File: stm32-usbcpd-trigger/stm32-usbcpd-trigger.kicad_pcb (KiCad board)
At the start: 2 copper layers, 24.5 x 13.5 mm, 25 parts, among them J1 USB_C_Receptacle_USB2.0, J2 Conn_01x02_Socket, J3 VBUS, J4 GND, SW1 SW_Push, U1 FUSB302B01MPX, U2 STM32F030F4Px, U3 NCP718

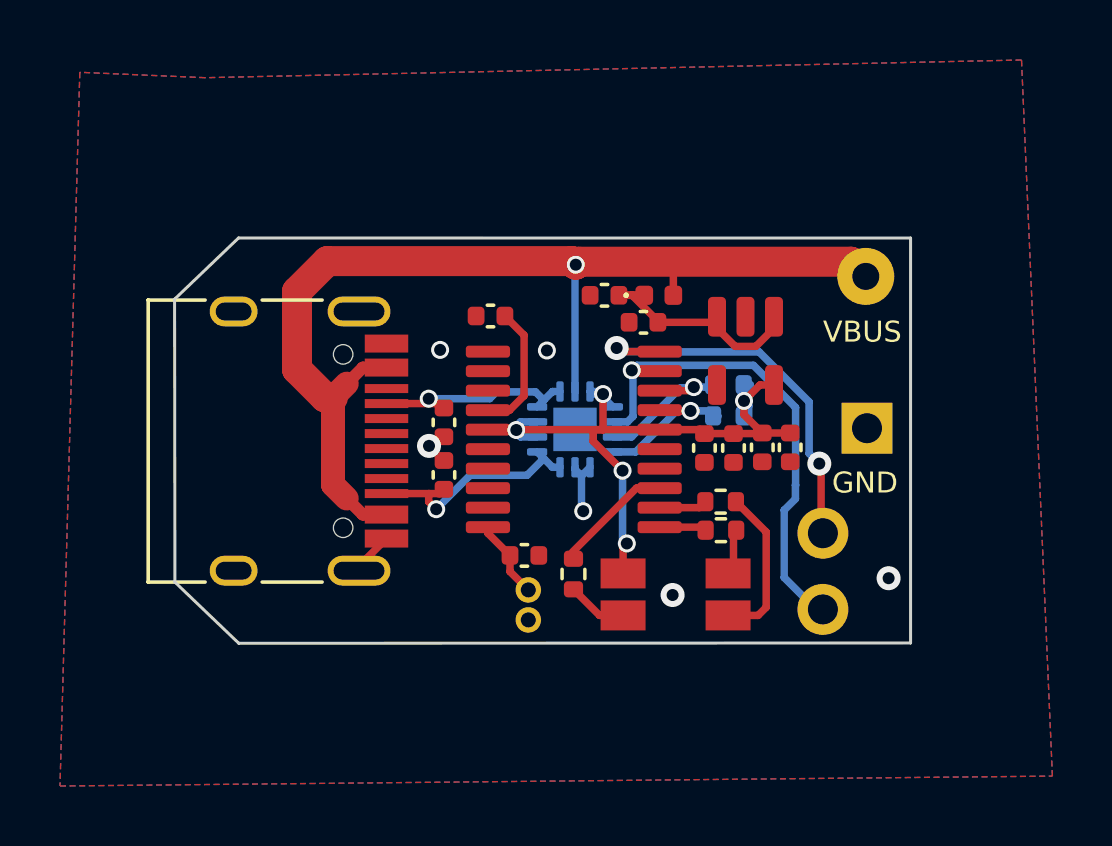
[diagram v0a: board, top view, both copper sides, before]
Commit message: updated stm32 trigger
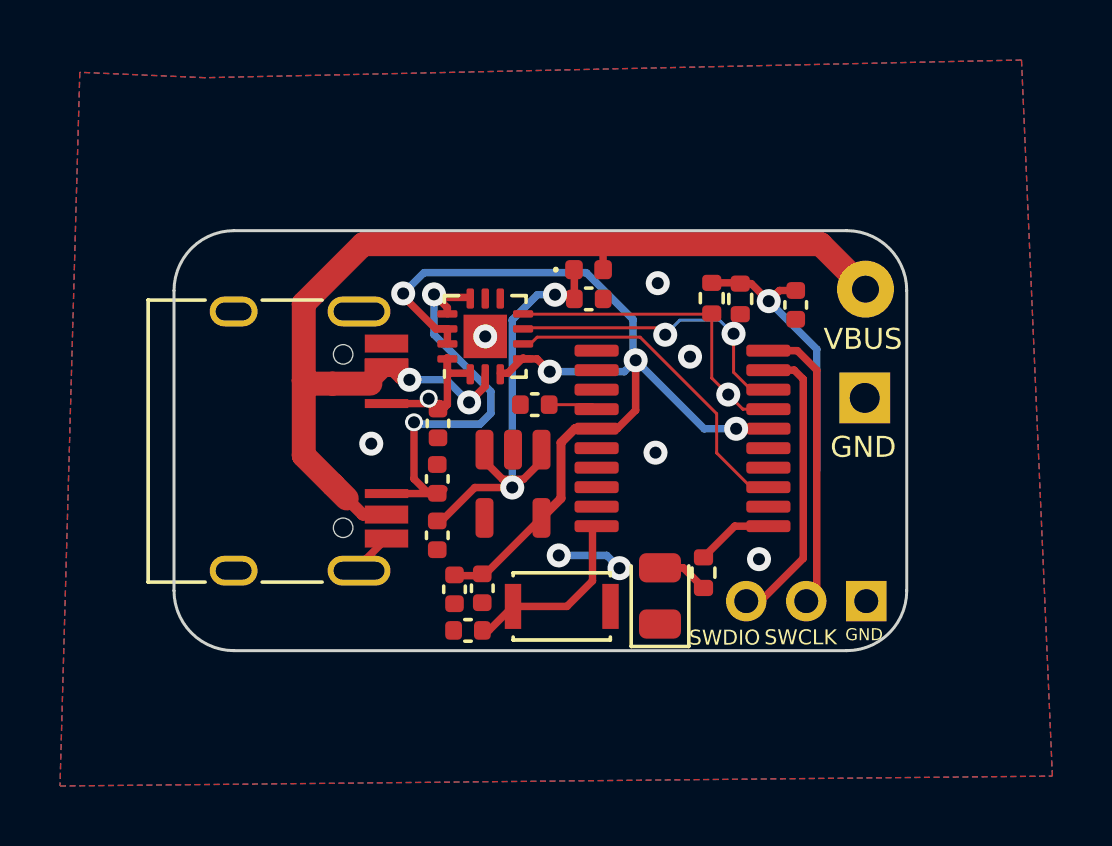
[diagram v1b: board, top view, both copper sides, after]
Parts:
- removed C4: 4.7uF, Capacitor_SMD:C_0402_1005Metric
- removed D3: LED_RGAB, LED_SMD:LED_RGB_1210
- removed R4, R6: 2.2k, Resistor_SMD:R_0402_1005Metric
- removed R5: 5.6k, Resistor_SMD:R_0402_1005Metric
- added D1: LED, LED_SMD:LED_0805_2012Metric, F.Cu at (130.9, 43.1)
- added R2: 3k, Resistor_SMD:R_0402_1005Metric, F.Cu at (132.3, 42.4)
- J2: footprint Connector_PinSocket_2.54mm:PinSocket_1x02_P2.54mm_Vertical -> Connector_PinHeader_2.00mm:PinHeader_1x03_P2.00mm_Vertical
- R1, R3, U1: moved to F.Cu
- SW1: footprint Connector_PinHeader_1.00mm:PinHeader_1x02_P1.00mm_Vertical -> Button_Switch_SMD:SW_SPST_CK_KXT3
- moved C5 11.3 mm to (124.0, 42.9)
- moved C9 11.3 mm to (125.0, 42.9)
- moved C3 9.75 mm to (123.5, 41.1), turned to -90 degrees
- moved U3 8.93 mm to (126.0, 39.4)
- moved C10 5.66 mm to (135.4, 33.5), turned to 90 degrees
- moved U1 4.31 mm to (125.1, 34.5), turned to 90 degrees
- moved R3 3.96 mm to (132.6, 33.2), turned to 90 degrees
- moved U2 3.62 mm to (131.7, 37.9)
- moved C1 3.30 mm to (126.7, 36.8)
- moved C6 3.13 mm to (124.5, 44.3), turned to 180 degrees
- moved R1 2.89 mm to (133.6, 33.2), turned to 90 degrees
- moved J2 2.69 mm to (137.8, 43.3), turned to -90 degrees
- moved D4 2.49 mm to (128.5, 32.3)
- moved C2 1.98 mm to (128.5, 33.2), turned to 0 degrees
- moved SW1 1.20 mm to (127.6, 43.5)
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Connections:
- C10 pad 1: +3V3 -> GND
- C10 pad 2: GND -> +3V3
- J2 pad 1: /SWCLK -> GND
- J2 pad 2: /INTN -> /SWCLK
- U2 pad 11: /LED_R -> /LED_PWR
- U2 pad 12: /LED_G -> unconnected-(U2-PA6-Pad12)
- U2 pad 13: /LED_B -> /INTN
- U2 pad 19: /INTN -> /SWDIO
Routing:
- net +3V3: track 24.5 -> 46.1 mm
- net /SWDIO: track 0.00 -> 9.75 mm
- net Net-(D4-K): track 8.20 -> 15.4 mm, vias 0 -> 2
- net Net-(J1-CC2): track 7.86 -> 14.1 mm, vias 1 -> 2
- net /INTN: track 16.9 -> 11.1 mm, vias 1 -> 0
- net /SDA: track 5.19 -> 10.8 mm
- net /SCL: track 5.47 -> 10.9 mm, vias 1 -> 2
- net Net-(D3-RK): track 5.32 -> 0.00 mm
- net /LED_B: track 3.82 -> 0.00 mm
- net /BTN: track 2.65 -> 6.42 mm
- net /SWCLK: track 13.4 -> 9.73 mm, vias 2 -> 0
- net Net-(U2-NRST): track 4.33 -> 1.64 mm
- net /LED_PWR: track 0.00 -> 2.59 mm
- net Net-(D3-BK): track 2.48 -> 0.00 mm
- net Net-(J1-CC1): track 7.16 -> 5.13 mm
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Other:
- board size 24.5 x 13.5 mm -> 24.4 x 14 mm
- board text added: "SWCLK"
- board text added: "SWDIO"

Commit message: added various wip projects
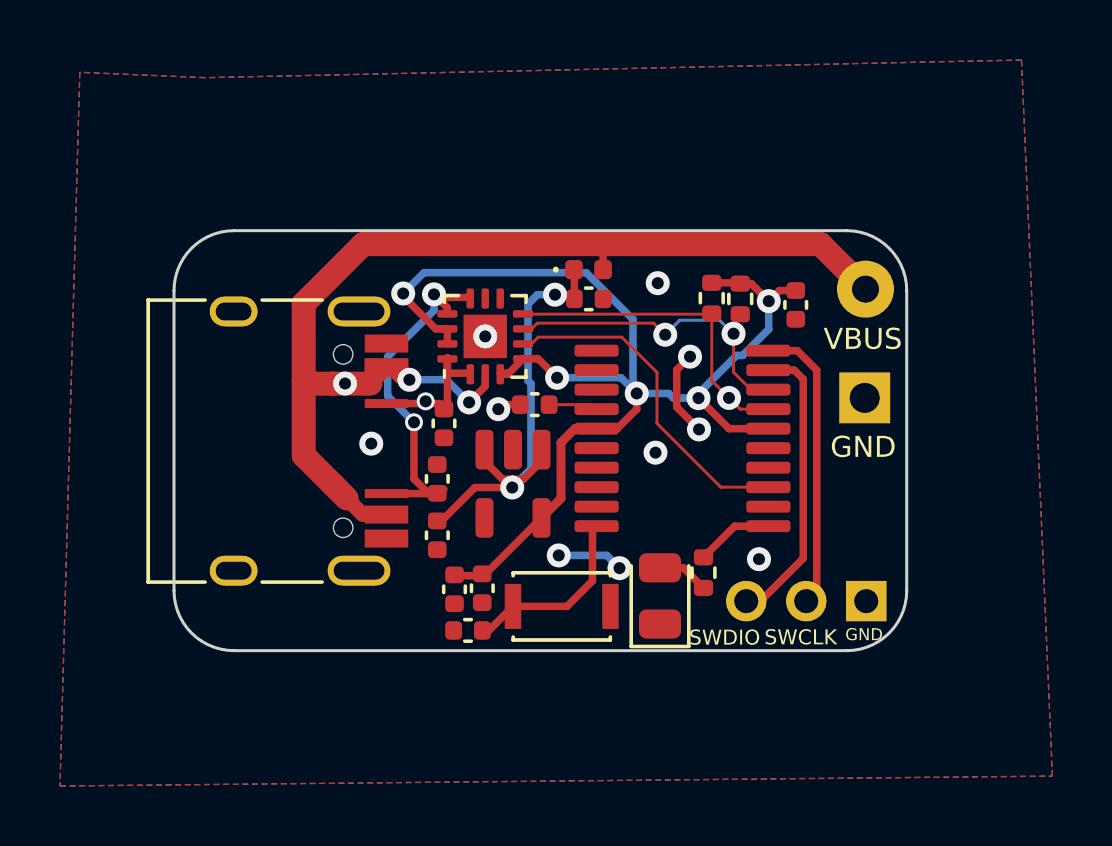
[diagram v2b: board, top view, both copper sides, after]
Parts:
- moved C7 0.20 mm to (123.7, 37.4)
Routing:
- net GND: track 4.79 -> 7.20 mm, vias 8 -> 10
- net Net-(J1-CC2): track 14.1 -> 11.9 mm
- net +3V3: track 46.1 -> 44.0 mm
- net /VBUS: track 38.1 -> 38.9 mm, vias 2 -> 3
